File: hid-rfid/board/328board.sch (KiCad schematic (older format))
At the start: 13 parts, among them IC1 ATTINY4313, J1 USB_2

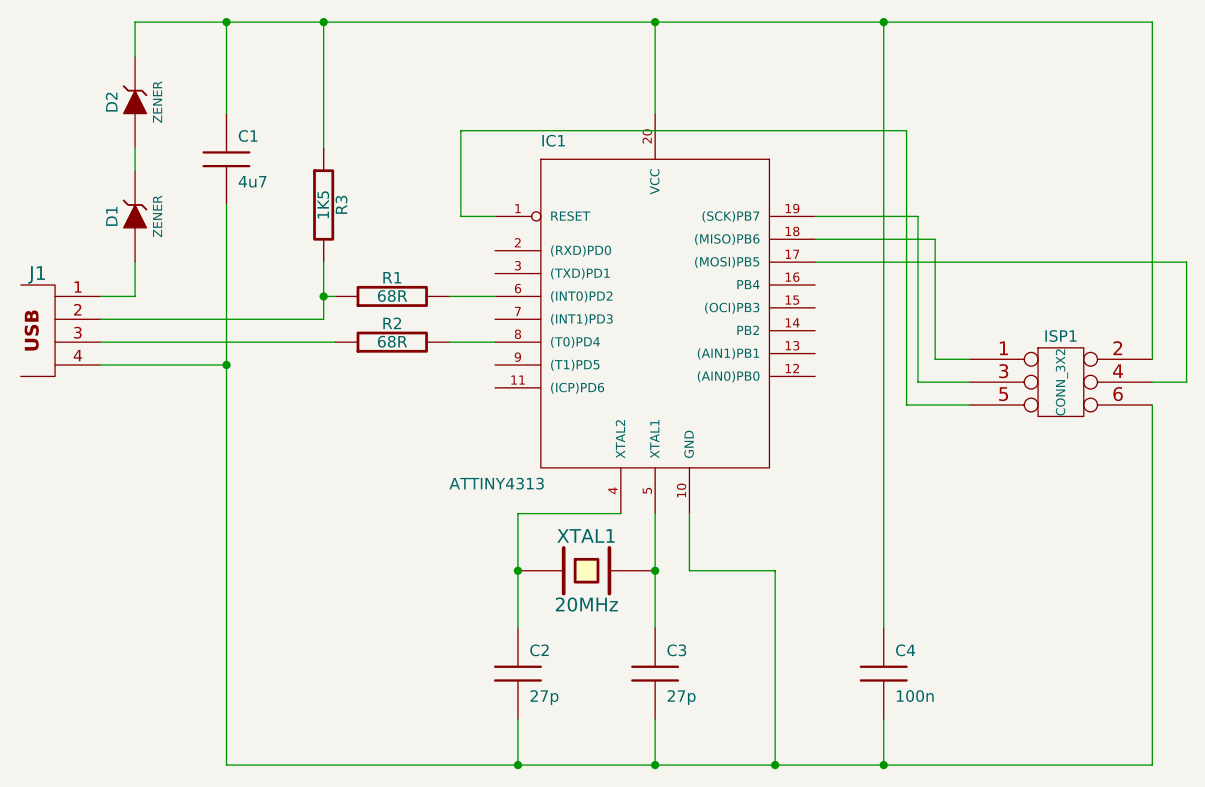
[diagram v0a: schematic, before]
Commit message: Novy board
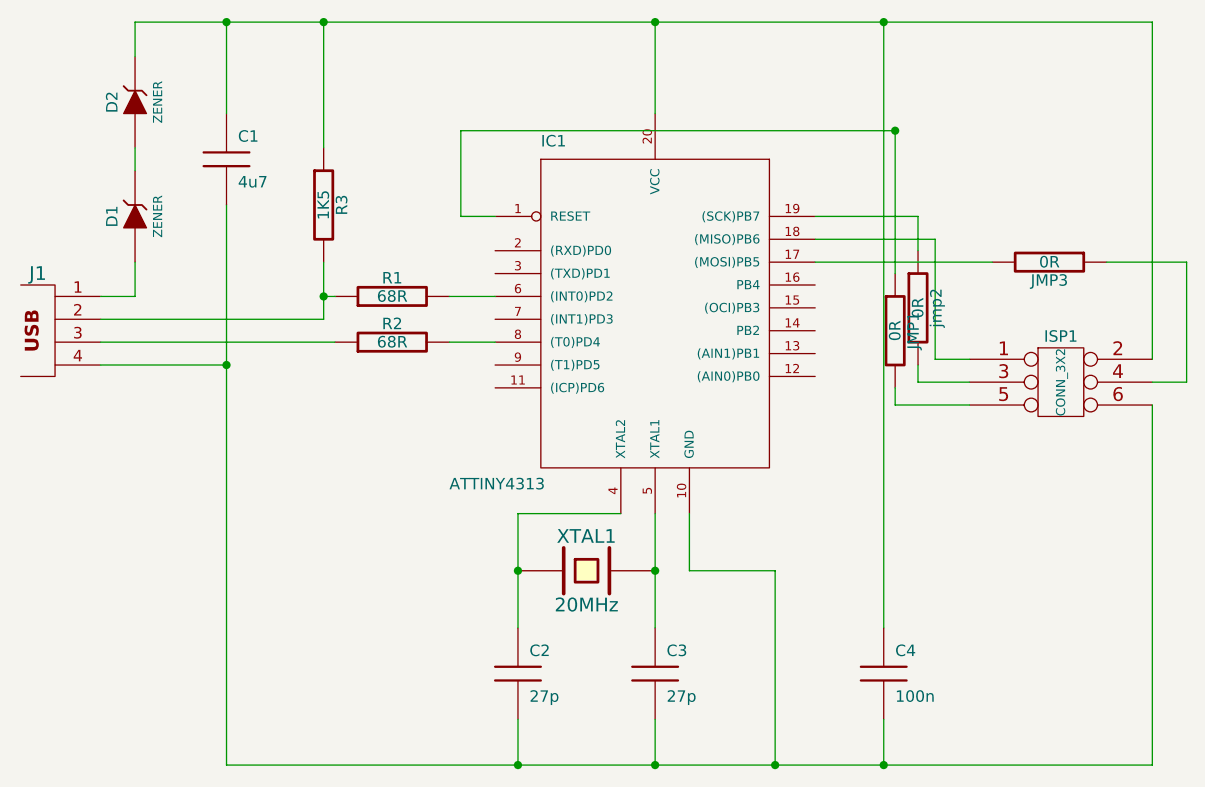
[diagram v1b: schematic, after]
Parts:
- added JMP1, JMP3, jmp2: 0R, symbol R
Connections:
- net at IC1.1 (RESET): now also JMP1.1; no longer ISP1.5
- net at IC1.17 ((MOSI)PB5): now also JMP3.2; no longer ISP1.4
- net at IC1.19 ((SCK)PB7): now also jmp2.1; no longer ISP1.3
- new net: ISP1.3, jmp2.2
- new net: ISP1.4, JMP3.1
- new net: ISP1.5, JMP1.2
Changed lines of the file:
@@
-EESchema Schematic File Version 2  date Ut 14. október 2014, 14:14:01 CEST
+EESchema Schematic File Version 2  date St 15. október 2014, 12:28:05 CEST
 LIBS:power
 LIBS:device
@@
 Sheet 1 1
 Title ""
-Date "14 oct 2014"
+Date "15 oct 2014"
 Rev ""
 Comp ""
@@
 $EndDescr
 Wire Wire Line
-	4200 2000 5825 2000
+	5475 2000 5825 2000
+Wire Wire Line
+	4650 1950 4650 1800
+Wire Wire Line
+	4875 2625 4550 2625
+Wire Wire Line
+	4550 2625 4550 2550
+Connection ~ 4550 1425
+Wire Wire Line
+	4550 2050 4550 1425
+Wire Wire Line
+	5675 2525 5825 2525
+Wire Wire Line
+	5825 2525 5825 2000
+Connection ~ 4500 4200
+Wire Wire Line
+	5675 2625 5675 4200
+Wire Wire Line
+	5675 4200 1625 4200
+Wire Wire Line
+	4875 2525 4650 2525
+Wire Wire Line
+	4650 1800 4200 1800
+Connection ~ 3500 950
+Wire Wire Line
+	4500 950  4500 3600
+Connection ~ 4025 4200
+Wire Wire Line
+	4025 4200 4025 3350
+Wire Wire Line
+	4025 3350 3650 3350
+Wire Wire Line
+	3650 3350 3650 3100
+Wire Wire Line
+	3500 4200 3500 4000
+Wire Wire Line
+	2900 4200 2900 4000
+Connection ~ 2900 3350
+Wire Wire Line
+	2900 3600 2900 3100
+Wire Wire Line
+	2900 3100 3350 3100
+Connection ~ 1625 950
+Wire Wire Line
+	1625 1350 1625 950
+Wire Wire Line
+	2100 2350 1075 2350
+Connection ~ 2050 950
+Wire Wire Line
+	2050 1500 2050 950
+Wire Wire Line
+	2050 2150 2100 2150
+Wire Wire Line
+	3500 950  3500 1350
+Wire Wire Line
+	1225 1100 1225 950
+Wire Wire Line
+	1225 2000 1225 2150
+Wire Wire Line
+	1225 2150 1075 2150
+Wire Wire Line
+	2600 2350 2800 2350
+Wire Wire Line
+	2600 2150 2800 2150
+Wire Wire Line
+	1225 1600 1225 1500
+Wire Wire Line
+	2050 2000 2050 2250
+Connection ~ 2050 2150
+Wire Wire Line
+	2050 2250 1075 2250
+Wire Wire Line
+	1625 2450 1075 2450
+Wire Wire Line
+	3500 3600 3500 3100
+Connection ~ 3500 3350
+Wire Wire Line
+	4500 4200 4500 4000
+Connection ~ 3500 4200
+Wire Wire Line
+	1625 4200 1625 1750
+Connection ~ 2900 4200
+Connection ~ 1625 2450
+Wire Wire Line
+	4200 1900 4725 1900
+Wire Wire Line
+	4725 1900 4725 2425
+Wire Wire Line
+	4725 2425 4875 2425
+Wire Wire Line
+	2800 1800 2650 1800
+Wire Wire Line
+	2650 1800 2650 1425
+Wire Wire Line
+	1225 950  5675 950
+Wire Wire Line
+	5675 950  5675 2425
 Connection ~ 4500 950
 Wire Wire Line
-	5675 2425 5675 950
-Wire Wire Line
-	5675 950  1225 950
-Wire Wire Line
-	4875 2625 4600 2625
-Wire Wire Line
-	4600 2625 4600 1425
-Wire Wire Line
-	4600 1425 2650 1425
-Wire Wire Line
-	2650 1425 2650 1800
-Wire Wire Line
-	2650 1800 2800 1800
-Wire Wire Line
-	4875 2425 4725 2425
-Wire Wire Line
-	4725 2425 4725 1900
-Wire Wire Line
-	4725 1900 4200 1900
-Connection ~ 1625 2450
-Connection ~ 2900 4200
-Wire Wire Line
-	1625 1750 1625 4200
-Connection ~ 3500 4200
-Wire Wire Line
-	4500 4200 4500 4000
-Connection ~ 3500 3350
-Wire Wire Line
-	3500 3600 3500 3100
-Wire Wire Line
-	1625 2450 1075 2450
-Wire Wire Line
-	1075 2250 2050 2250
-Connection ~ 2050 2150
-Wire Wire Line
-	2050 2250 2050 2000
-Wire Wire Line
-	1225 1600 1225 1500
-Wire Wire Line
-	2600 2150 2800 2150
-Wire Wire Line
-	2600 2350 2800 2350
-Wire Wire Line
-	1075 2150 1225 2150
-Wire Wire Line
-	1225 2150 1225 2000
-Wire Wire Line
-	1225 950  1225 1100
-Wire Wire Line
-	3500 950  3500 1350
-Wire Wire Line
-	2050 2150 2100 2150
-Wire Wire Line
-	2050 1500 2050 950
-Connection ~ 2050 950
-Wire Wire Line
-	2100 2350 1075 2350
-Wire Wire Line
-	1625 1350 1625 950
-Connection ~ 1625 950
-Wire Wire Line
-	3350 3100 2900 3100
-Wire Wire Line
-	2900 3100 2900 3600
-Connection ~ 2900 3350
-Wire Wire Line
-	2900 4200 2900 4000
-Wire Wire Line
-	3500 4200 3500 4000
-Wire Wire Line
-	3650 3100 3650 3350
-Wire Wire Line
-	3650 3350 4025 3350
-Wire Wire Line
-	4025 3350 4025 4200
-Connection ~ 4025 4200
-Wire Wire Line
-	4500 950  4500 3600
-Connection ~ 3500 950
-Wire Wire Line
-	4200 1800 4650 1800
-Wire Wire Line
-	4650 1800 4650 2525
-Wire Wire Line
-	4650 2525 4875 2525
-Wire Wire Line
-	1625 4200 5675 4200
-Wire Wire Line
-	5675 4200 5675 2625
-Connection ~ 4500 4200
-Wire Wire Line
-	5825 2000 5825 2525
-Wire Wire Line
-	5825 2525 5675 2525
-$Comp
-L CONN_3X2 ISP1
-U 1 1 543D11D8
-P 5275 2575
-F 0 "ISP1" H 5275 2825 50  0000 C CNN
-F 1 "CONN_3X2" V 5275 2625 40  0000 C CNN
-	1    5275 2575
-	1    0    0    -1
-$EndComp
+	2650 1425 4550 1425
+Wire Wire Line
+	4650 2525 4650 2450
+Wire Wire Line
+	4200 2000 4975 2000
 $Comp
 L USB_2 J1
@@
 	1    0    0    -1
 $EndComp
+$Comp
+L R JMP3
+U 1 1 543E4AE0
+P 5225 2000
+F 0 "JMP3" V 5305 2000 50  0000 C CNN
+F 1 "0R" V 5225 2000 50  0000 C CNN
+	1    5225 2000
+	0    1    1    0
+$EndComp
+$Comp
+L R jmp2
+U 1 1 543E4ADC
+P 4650 2200
+F 0 "jmp2" V 4730 2200 50  0000 C CNN
+F 1 "0R" V 4650 2200 50  0000 C CNN
+	1    4650 2200
+	1    0    0    -1
+$EndComp
+$Comp
+L R JMP1
+U 1 1 543E4AD9
+P 4550 2300
+F 0 "JMP1" V 4630 2300 50  0000 C CNN
+F 1 "0R" V 4550 2300 50  0000 C CNN
+	1    4550 2300
+	1    0    0    -1
+$EndComp
+$Comp
+L CONN_3X2 ISP1
+U 1 1 543D11D8
+P 5275 2575
+F 0 "ISP1" H 5275 2825 50  0000 C CNN
+F 1 "CONN_3X2" V 5275 2625 40  0000 C CNN
+	1    5275 2575
+	1    0    0    -1
+$EndComp
